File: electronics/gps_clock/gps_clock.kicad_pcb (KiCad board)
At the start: 4 copper layers, 218.5 x 71 mm, 134 parts, among them J1 USB_C_Receptacle_PowerOnly_24P, J2 TC2030, Q10 BSS127S, Q11 BSS127S, Q12 BSS127S, Q13 BSS127S, Q14 BSS127S, Q15 BSS127S, Q16 BSS127S, Q17 BSS127S, Q18 BSS127S, Q19 BSS127S, Q2 FDS2672CT, Q20 BSS127S, Q21 BSS127S, Q22 BSS127S, Q23 BSS127S, Q24 BSS127S, Q25 BSS127S, Q26 BSS127S, Q27 BSS127S, Q28 BSS127S, Q29 BSS127S, Q3 BSS127S, Q30 BSS127S, Q31 BSS127S, Q32 BSS127S, Q33 BSS127S, Q34 BSS127S, Q35 BSS127S, Q36 BSS127S, Q37 BSS127S, Q38 BSS127S, Q39 BSS127S, Q4 BSS127S, Q40 BSS127S, Q41 BSS127S, Q42 BSS127S, Q43 BSS127S, Q44 BSS127S, Q45 BSS127S, Q46 BSS127S, Q47 BSS127S, Q48 BSS127S, Q49 BSS127S, Q5 BSS127S, Q50 BSS127S, Q51 BSS127S, Q52 BSS127S, Q53 BSS127S, Q54 BSS127S, Q55 BSS127S, Q56 BSS127S, Q57 BSS127S, Q58 BSS127S, Q59 BSS127S, Q6 BSS127S, Q60 BSS127S, Q61 BSS127S, Q62 BSS127S, Q7 BSS127S, Q8 BSS127S, Q9 BSS127S, SW1 SW_Push, U1 MIC5365-3.3YD5, U10 74HC595, U11 74HC595, U12 74HC595, U2 PA1616D, U3 STM32G070RBTx, U4 UCC3803, U5 74HC595, U6 74HC595, U7 74HC595, U8 74HC595, U9 74HC595, X1 32kHz768

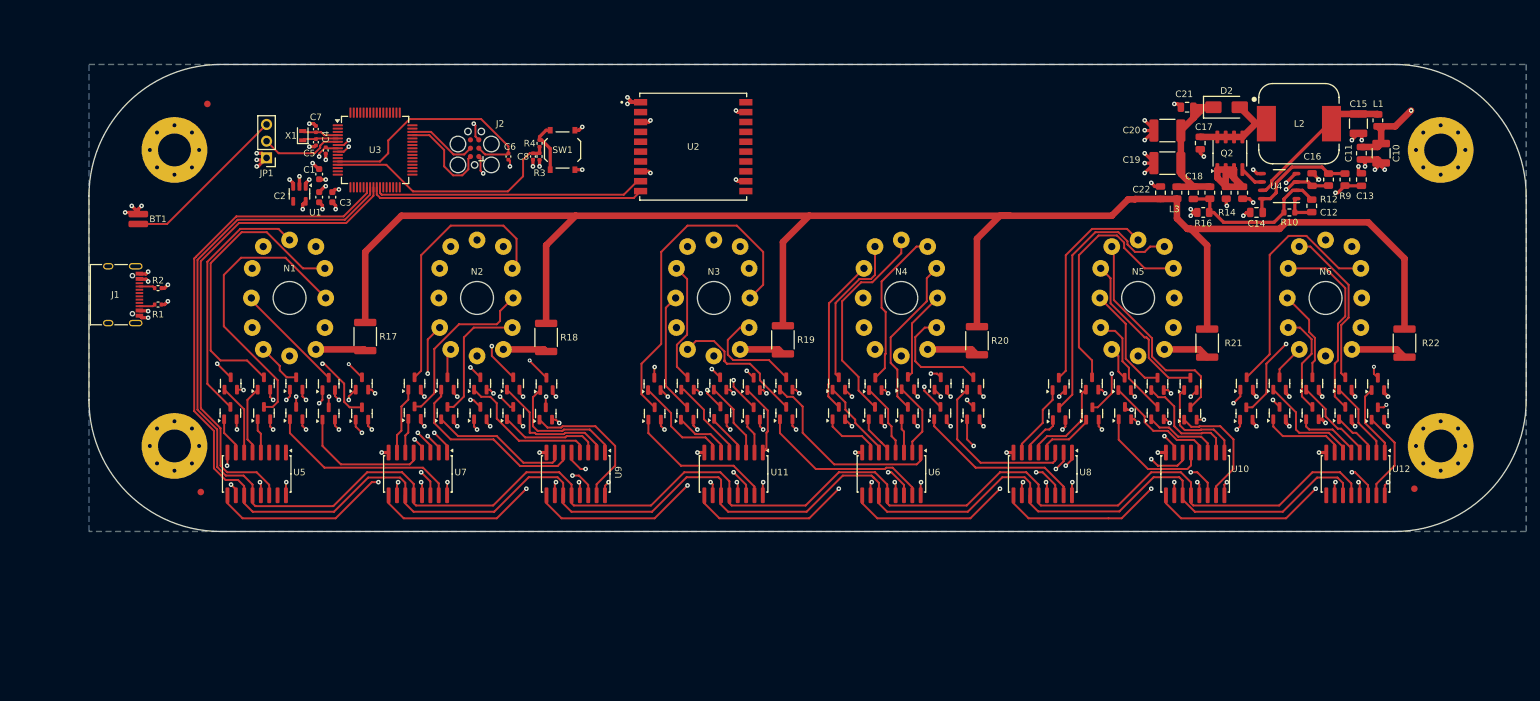
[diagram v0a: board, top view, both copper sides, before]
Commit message: updated pcb
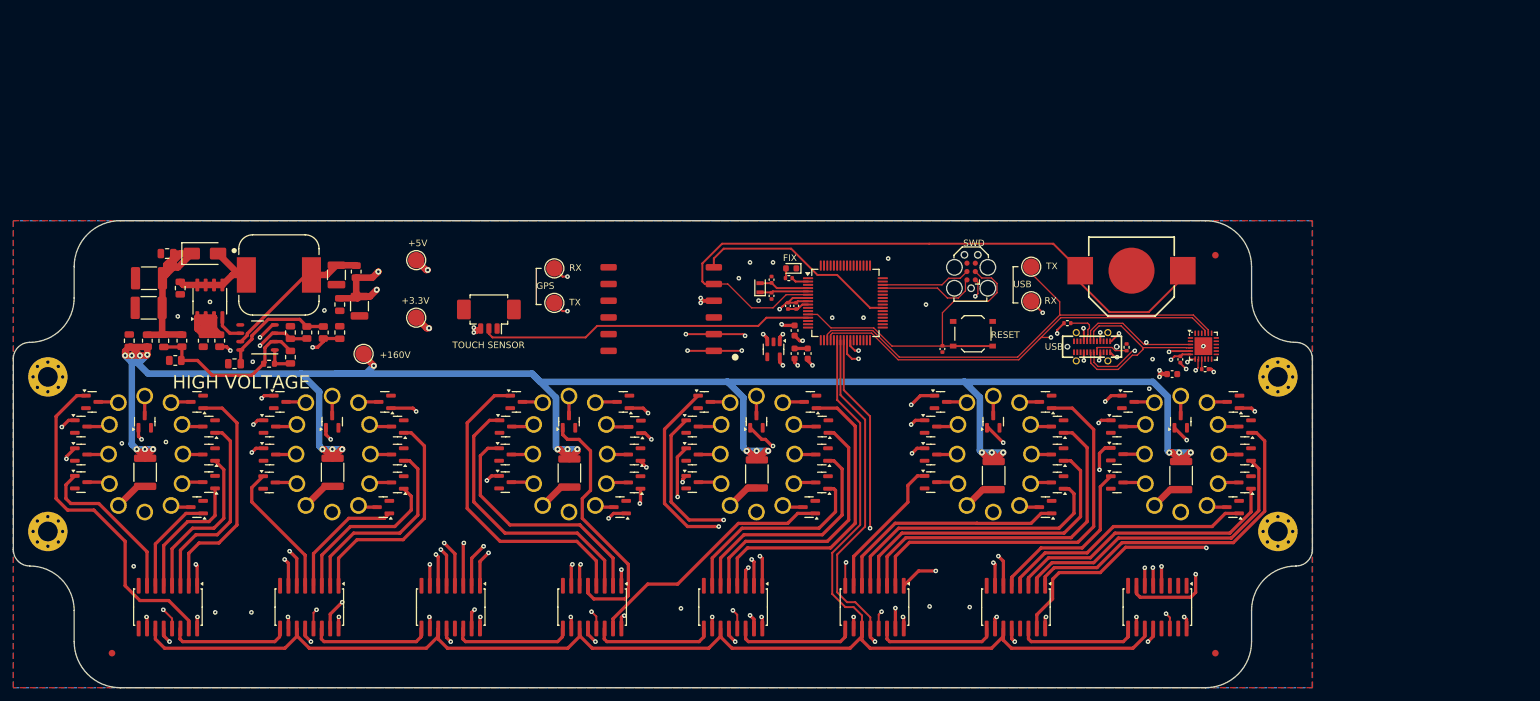
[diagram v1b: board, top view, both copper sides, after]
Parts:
- removed BT1: Battery_Cell, Library:MS518SE-FL35E
- removed C8: 100n, Capacitor_SMD:C_0402_1005Metric
- removed JP1: Jumper_3_Open, Connector_PinHeader_2.54mm:PinHeader_1x03_P2.54mm_Vertical
- removed R3: 5k1, Resistor_SMD:R_0402_1005Metric
- removed R4: 100R, Resistor_SMD:R_0402_1005Metric
- removed SW1: SW_Push, Button_Switch_SMD:SW_Push_1P1T_XKB_TS-1187A
- added BT2: ~, Library:BAT-SMD_MY-1220-03, F.Cu at (255.0, 143.8)
- added C23: 100n, Capacitor_SMD:C_0402_1005Metric, F.Cu at (262.4, 157.3)
- added C24: 4u7, Capacitor_SMD:C_0603_1608Metric, F.Cu at (261.2, 159.6)
- added C9: 100n, Capacitor_SMD:C_0402_1005Metric, F.Cu at (202.8, 149.2)
- added D1: LED, Diode_SMD:D_0603_1608Metric, F.Cu at (203.2, 143.5)
- added J3: USB_C_Receptacle_USB2.0_14P, Library:USB-C-SMD_U263-241N-4BQC02, F.Cu at (249.0, 155.4)
- added R5: 5k1, Resistor_SMD:R_0402_1005Metric, F.Cu at (254.2, 155.5)
- added R6: 5k1, Resistor_SMD:R_0402_1005Metric, F.Cu at (245.2, 151.8)
- added SW2: SW_Push, Button_Switch_SMD:SW_Push_1P1T_XKB_TS-1187A, F.Cu at (230.9, 153.4)
- added TP1: TestPoint, TestPoint:TestPoint_Pad_D2.5mm, F.Cu at (146.2, 151.0)
- added TP2: TestPoint, TestPoint:TestPoint_Pad_D2.5mm, F.Cu at (146.2, 142.2)
- added TP3: TestPoint, TestPoint:TestPoint_Pad_D2.5mm, F.Cu at (138.2, 156.5)
- added TP4: TestPoint, TestPoint:TestPoint_Pad_D2.5mm, F.Cu at (167.2, 143.5)
- added TP5: TestPoint, TestPoint:TestPoint_Pad_D2.5mm, F.Cu at (167.2, 148.8)
- added TP6: TestPoint, TestPoint:TestPoint_Pad_D2.5mm, F.Cu at (239.8, 143.2)
- added TP7: TestPoint, TestPoint:TestPoint_Pad_D2.5mm, F.Cu at (239.8, 148.5)
- added U13: TU10-F, Library:TU10-F, F.Cu at (183.5, 149.8)
- H1, H2, H3, H4: value MountingHole -> MountingHole_Pad; footprint MountingHole:MountingHole_5mm_Pad_Via -> MountingHole:MountingHole_3mm_Pad_Via
- J1: value USB_C_Receptacle_PowerOnly_24P -> Conn_01x03_Pin; footprint Connector_USB:USB_C_Receptacle_XKB_U262-16XN-4BVC11 -> Connector_Molex:Molex_PicoBlade_53261-0371_1x03-1MP_P1.25mm_Horizontal
- N1, N2, N3, N4, N5, N6: moved to B.Cu
- R1: value 5k1 -> 10k
- U2: value PA1616D -> CP2104; footprint Library:CD-PA1616D_ADA -> Package_DFN_QFN:QFN-24-1EP_4x4mm_P0.5mm_EP2.7x2.7mm
- moved Q31 195.5 mm to (97.0, 163.8), turned to 0 degrees
- moved R22 192.5 mm to (105.0, 174.5)
- moved Q27 187.6 mm to (105.0, 166.8)
- moved Q3 182.5 mm to (95.3, 176.0), turned to 0 degrees
- moved U12 181.7 mm to (108.5, 195.0)
- moved N6 181.1 mm to (105.0, 171.7), turned to 180 degrees
- moved Q35 177.3 mm to (95.3, 167.6), turned to 0 degrees
- moved Q39 177.3 mm to (95.3, 171.8), turned to 0 degrees
- moved Q23 174.6 mm to (112.9, 163.8), turned to 180 degrees
- moved Q19 172.8 mm to (114.7, 167.6), turned to 180 degrees
- moved Q15 168.1 mm to (114.7, 171.8), turned to 180 degrees
- moved Q11 168.1 mm to (114.7, 176.0), turned to 180 degrees
- moved Q7 165.7 mm to (112.9, 179.8), turned to 180 degrees
- moved R1 159.5 mm to (266.2, 158.8), turned to 180 degrees
- moved FM1 158.4 mm to (267.8, 141.5)
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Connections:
- H1 pad 1: (no net) -> GND
- H2 pad 1: (no net) -> GND
- H3 pad 1: (no net) -> GND
- H4 pad 1: (no net) -> GND
- R1 pad 1: Net-(J1-CC2) -> +3.3V
- R1 pad 2: GND -> Net-(U2-~{RST})
- R2 pad 1: Net-(J1-CC1) -> /GPS_FIX
- R2 pad 2: GND -> Net-(D1-A)
- U2 pad 1: +3.3V -> unconnected-(U2-~{RI}-Pad1)
- U2 pad 10: /USART1_TX -> unconnected-(U2-NC-Pad10)
- U2 pad 12: GND -> unconnected-(U2-RS485/GPIO.2-Pad12)
- U2 pad 19: GND -> unconnected-(U2-~{RTS}-Pad19)
- U2 pad 2: unconnected-(U2-NRST-Pad2) -> GND
- U2 pad 20: unconnected-(U2-NC-Pad20) -> /USART2_TX
- U2 pad 3: GND -> /D+
- U2 pad 4: unconnected-(U2-VBACKUP-Pad4) -> /D-
- U2 pad 5: unconnected-(U2-3D-FIX-Pad5) -> +3.3V
- U2 pad 6: unconnected-(U2-NC-Pad6) -> +3.3V
- U2 pad 7: unconnected-(U2-NC-Pad7) -> +3.3V
- U2 pad 8: GND -> +5V
- U2 pad 9: /USART1_RX -> Net-(U2-~{RST})
- U3 pad 13: Net-(U3-PC0) -> Net-(J1-Pin_2)
- U3 pad 19: unconnected-(U3-PA2-Pad19) -> /USART2_TX
- U3 pad 2: unconnected-(U3-PC12-Pad2) -> /GPS_FIX
- U3 pad 20: unconnected-(U3-PA3-Pad20) -> /USART2_RX
- U3 pad 39: unconnected-(U3-PC7-Pad39) -> /1PPS
- U3 pad 6: Net-(JP1-C) -> /VBAT
- U3 pad 7: GND -> +3.3V
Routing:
- net GND: track 181.7 -> 32.6 mm, vias 122 -> 34
- net /VBAT: track 0.00 -> 104.2 mm
- net /USART2_TX: track 0.00 -> 74.0 mm
- net /USART2_RX: track 0.00 -> 72.0 mm, vias 0 -> 2
- net /LATCH: track 281.0 -> 217.4 mm, vias 0 -> 8
- net /SPI_CLK: track 283.1 -> 228.4 mm
- net Net-(J1-Pin_2): track 0.00 -> 50.8 mm
- net /Nixie Tube Driver/B18: track 6.72 -> 56.3 mm, vias 0 -> 2
- net /Nixie Tube Driver/IN3-9: track 52.3 -> 3.35 mm
- net +160V: track 262.3 -> 309.8 mm, vias 0 -> 23
- net /Nixie Tube Driver/IN1-8: track 44.7 -> 3.52 mm
- net /Nixie Tube Driver/IN1-9: track 44.2 -> 3.27 mm
- net /Nixie Tube Driver/B36: track 6.61 -> 46.1 mm
- net /Nixie Tube Driver/B46: track 20.3 -> 59.0 mm
- net /Nixie Tube Driver/IN5-7: track 41.3 -> 3.05 mm
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- added copper zone on F.Cu, net GND
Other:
- board size 218.5 x 71 mm -> 197.5 x 71 mm
- board text added: "+160V"
- board text added: "+3.3V"
- board text added: "+5V"
- board text added: "FIX"
- board text added: "GPS"
- board text added: "HIGH VOLTAGE"
- board text added: "RESET"
- board text added: "RX"
- board text added: "SWD"
- board text added: "TOUCH SENSOR"
- board text added: "TX"
- board text added: "USB"

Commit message: updated pcb
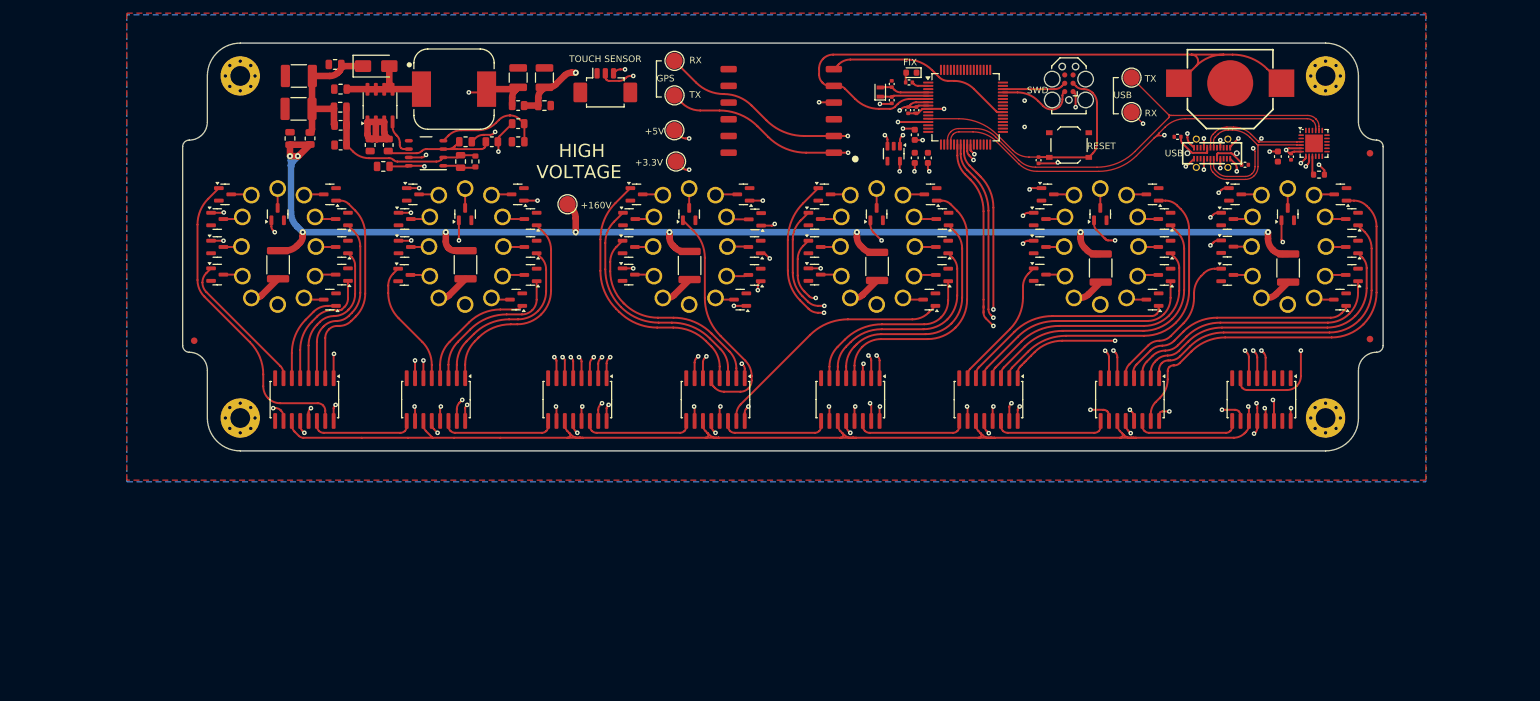
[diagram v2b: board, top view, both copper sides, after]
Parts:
- R1: footprint Resistor_SMD:R_0402_1005Metric -> Resistor_SMD:R_0603_1608Metric
- moved H1 54.3 mm to (119.5, 114.2)
- moved FM2 53.2 mm to (291.2, 154.2)
- moved FM3 49.1 mm to (112.5, 154.5)
- moved H2 46.3 mm to (284.5, 114.2)
- moved TP1 46.1 mm to (185.8, 127.2)
- moved C10 44.7 mm to (165.8, 114.5), turned to 90 degrees
- moved C18 44.5 mm to (134.7, 119.0), turned to 0 degrees
- moved TP2 43.9 mm to (185.5, 122.5)
- moved R10 43.9 mm to (155.2, 127.2), turned to -90 degrees
- moved R9 43.4 mm to (161.8, 121.5), turned to 180 degrees
- moved C11 43.4 mm to (165.8, 118.8), turned to 0 degrees
- moved R16 41.3 mm to (134.8, 124.8)
- moved C15 40.8 mm to (161.8, 114.5), turned to 90 degrees
- moved R15 40.7 mm to (134.8, 121.8), turned to 0 degrees
- moved R12 40.4 mm to (157.8, 124.2), turned to 0 degrees
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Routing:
- net +160V: track 309.8 -> 205.7 mm, vias 23 -> 9
- net /SPI_CLK: track 228.4 -> 252.9 mm, vias 0 -> 2
- net /LATCH: track 217.4 -> 236.3 mm, vias 8 -> 10
- net /SPI_DATA: track 92.5 -> 77.5 mm
- net /Nixie Tube Driver/B10: track 57.5 -> 46.9 mm
- net /SWD_NRST: track 50.1 -> 40.1 mm
- net GND: track 32.6 -> 42.0 mm, vias 34 -> 19
- net /Nixie Tube Driver/B9: track 57.9 -> 48.7 mm
- net +5V: track 60.2 -> 69.3 mm, vias 29 -> 27
- net Net-(D2-K): track 31.9 -> 23.3 mm
- net /Nixie Tube Driver/B46: track 59.0 -> 50.6 mm
- net Net-(Q2-S-Pad1): track 21.5 -> 13.4 mm
- net /Nixie Tube Driver/B45: track 52.8 -> 45.1 mm
- net +3.3V: track 36.3 -> 28.7 mm, vias 14 -> 11
- net /Nixie Tube Driver/B18: track 56.3 -> 49.1 mm
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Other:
- board size 197.5 x 71 mm -> 182.5 x 62 mm
